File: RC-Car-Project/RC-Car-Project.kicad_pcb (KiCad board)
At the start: 4 copper layers, 80 x 120 mm, 180 parts, among them J1 Conn_01x02_Pin, J10 ANT_IF, J11 Conn_01x02, J12 Conn_01x02, J13 RF_IF, J14 Conn_01x02, J15 USB4120-03-C_REVA, J16 Conn_01x02, J2 Conn_01x02_Pin, J3 Conn_01x02_Pin, J4 Conn_01x02_Pin, J5 MCU_IF, J6 Conn_01x02, J7 Conn_01x02, J8 Conn_01x02, J9 Conn_02x09_Odd_Even, Q1 BTN8982TA, Q2 BTN8982TA, Q3 BTN8982TA, Q4 BTN8982TA, Q5 PMF250XNE, Q6 PMF250XNE, Q7 PMOS, Q8 PMF250XNE, Q9 PMF250XNE, SW1 SW_Push, SW2 SW_SPDT, U1 LMR16020PDDAR, U11 LMR16030PDDA, U3 STM32H743VGTx, U4 USBLC6-2SC6, U7 INA229AQDGSRQ1, U8 ADC082S021CIMM/NOPB, U9 SN74HC244PWR, Y1 Crystal

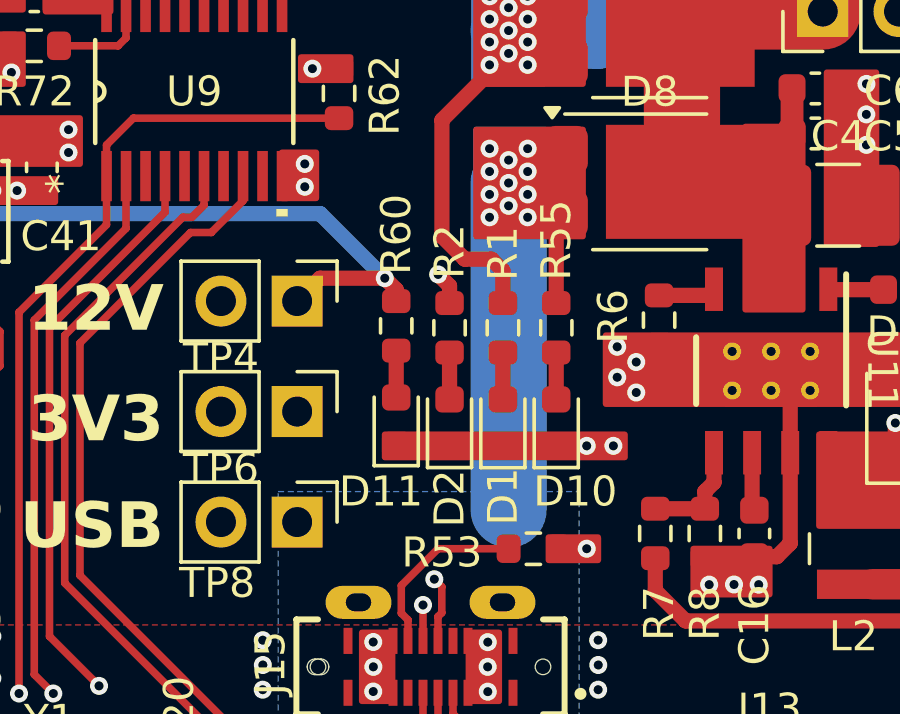
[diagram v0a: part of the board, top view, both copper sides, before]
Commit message: Fixed Bullshit
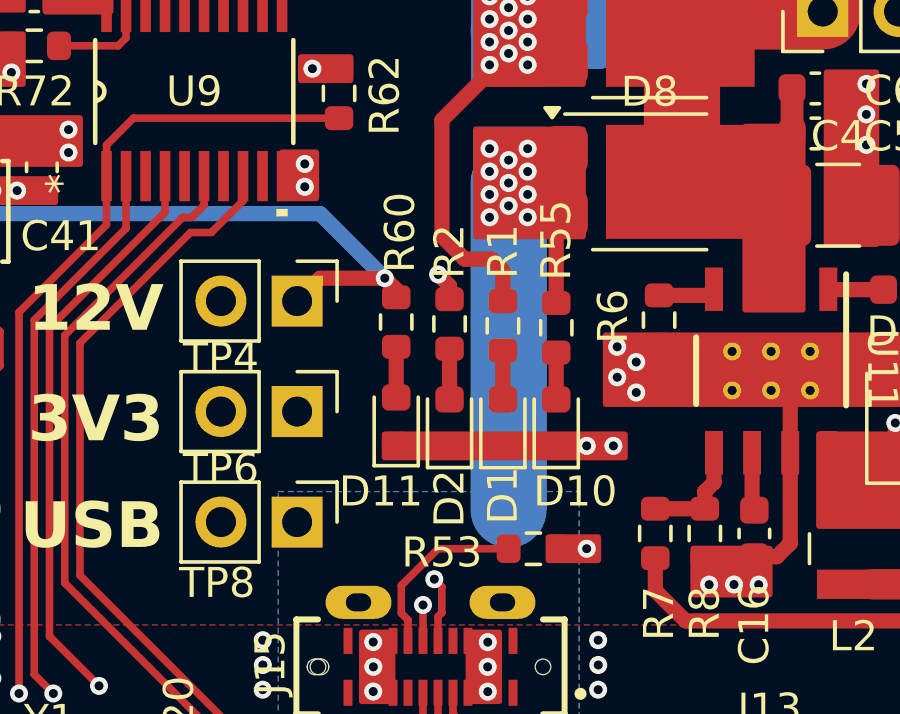
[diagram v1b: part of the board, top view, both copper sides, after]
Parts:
- C12: value 1uF/16V -> 1uF/10V
- C19, C31, C35: value 100nF/10V -> 0.1uF/10V
- C42, C45, C46, C47, C48: value 0.1uF/25V -> 0.1uF/10V
- R16, R21: value R -> 100kohm
- R20: value WSL27262L000FEB -> 0.002 OHM
- moved R2 0.13 mm to (165.6, 106.0)
- moved R60 0.13 mm to (163.8, 106.0)
- moved R1 0.06 mm to (167.4, 106.1)
